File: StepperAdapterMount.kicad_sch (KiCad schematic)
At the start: 4 parts, among them J1 Conn_01x04, M1 StepperMotor_4.7mm_Sanyo_ultr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

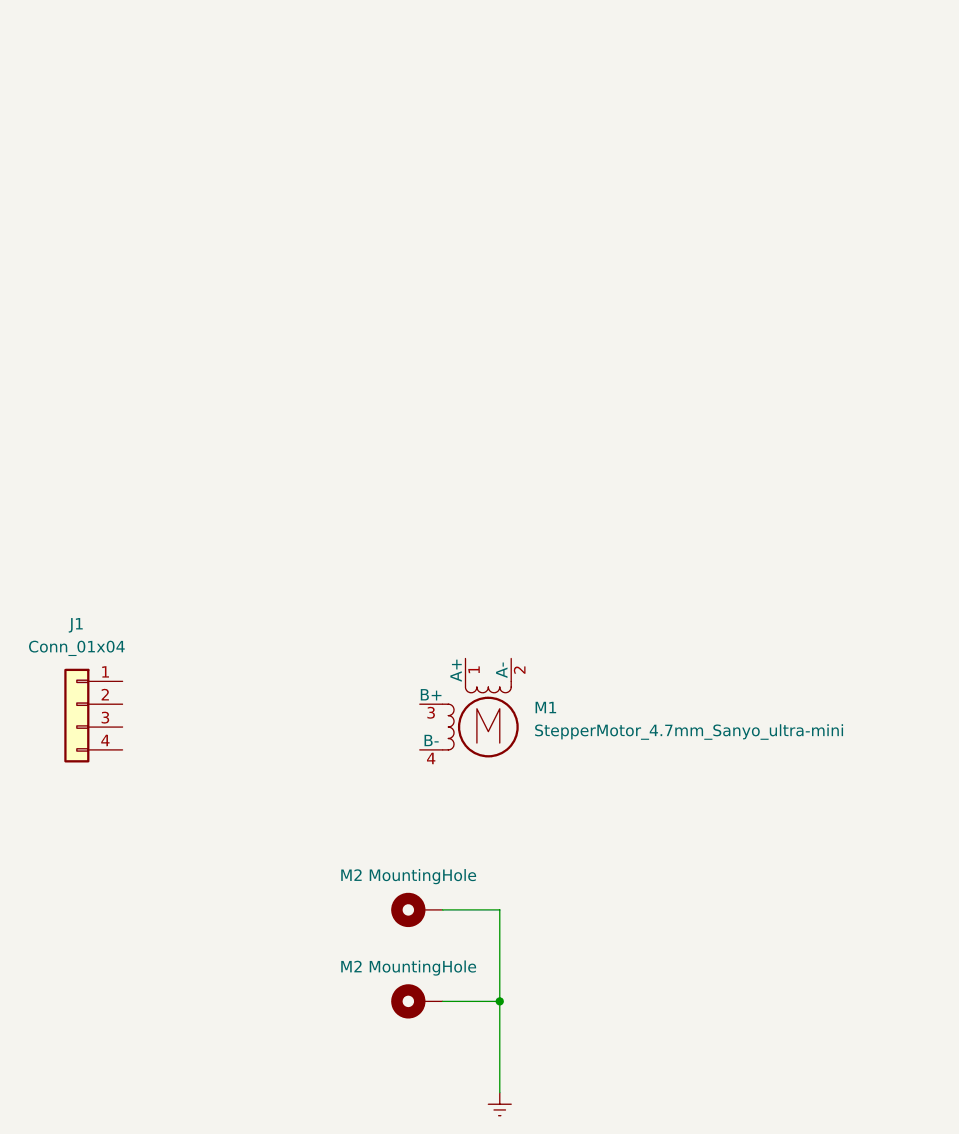
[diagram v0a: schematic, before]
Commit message: v1.0
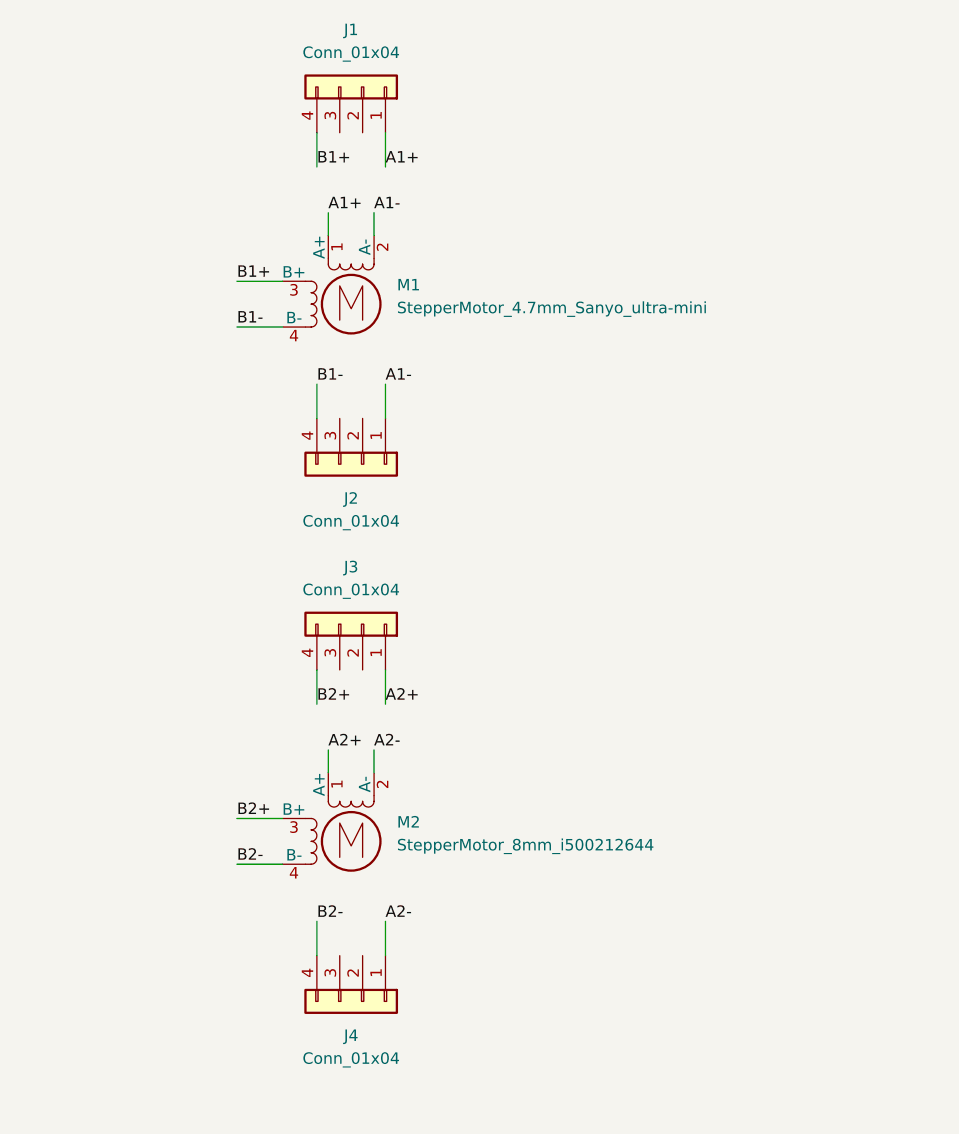
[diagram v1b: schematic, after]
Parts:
- removed H1, H2: M2 MountingHole, MountingHole:MountingHole_2.2mm_M2_ISO7380_Pad, symbol Mechanical:MountingHole_Pad
- added J2, J3, J4: Conn_01x04, Connector_PinHeader_2.54mm:PinHeader_1x04_P2.54mm_Vertical, symbol Connector_Generic:Conn_01x04
- added M2: StepperMotor_8mm_i500212644, AC-kicad-library:StepperMotor_8mm_i500212644, symbol AC-kicad-library:StepperMotor_8mm_i500212644
- J1: footprint Connector_Molex:Molex_PicoBlade_53261-0471_1x04-1MP_P1.25mm_Horizontal -> Connector_PinHeader_2.54mm:PinHeader_1x04_P2.54mm_Vertical
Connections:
- net A1+: now reaches M1.1 (A+)
- net A1+: now also J1.1 (Pin_1)
- net A1-: now reaches M1.2 (A-)
- net A1-: now also J2.1 (Pin_1)
- net B1+: now reaches M1.3 (B+)
- net B1+: now also J1.4 (Pin_4)
- net B1-: now reaches M1.4 (B-)
- net B1-: now also J2.4 (Pin_4)
- new net A2+: J3.1 (Pin_1), M2.1 (A+)
- new net A2-: J4.1 (Pin_1), M2.2 (A-)
- new net B2+: J3.4 (Pin_4), M2.3 (B+)
- new net B2-: J4.4 (Pin_4), M2.4 (B-)
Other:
- moved on the sheet: M1
